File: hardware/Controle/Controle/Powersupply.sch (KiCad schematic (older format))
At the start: 14 parts, among them U401 AMS1117-3.3, U402 AMS1117-5, U403 K78L15-1000R3

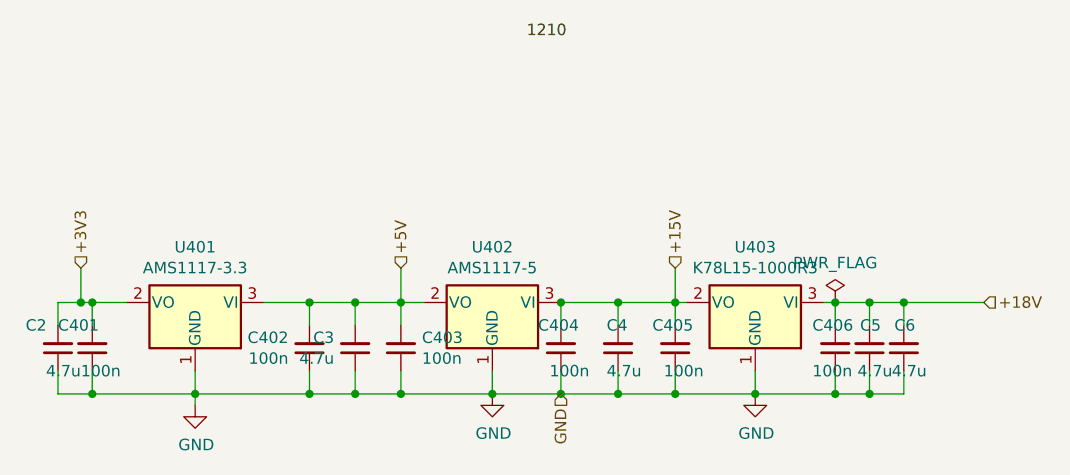
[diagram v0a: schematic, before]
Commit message: first version of layout
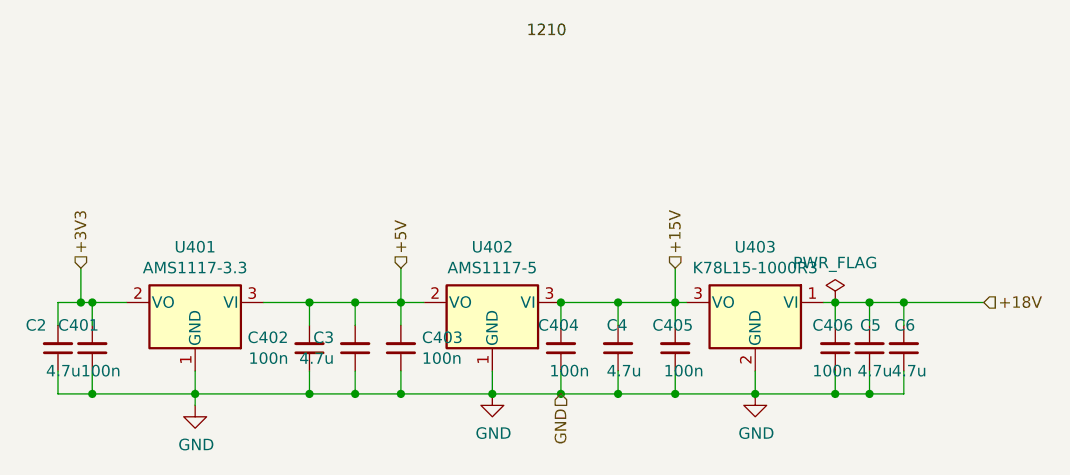
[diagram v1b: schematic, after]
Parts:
- removed U403: K78L15-1000R3, KicadZeniteSolarLibrary18:TO-220-3_Horizontal_TabDown_SMD, symbol Regulator_Linear:AP1117-15
- added U403: K78L15-1000R3, KicadZeniteSolarLibrary18:TO-220-3_Horizontal_Tabless_SMD, symbol Regulator_Linear:LM7805_TO220
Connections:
- net +15V: now also U403.3 (VO)
- net +18V: now also U403.1 (VI)
- net GND: now also U403.2 (GND)
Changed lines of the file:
@@
 GND
-$Comp
-L Regulator_Linear:AP1117-15 U403
-U 1 1 608AFF81
-P 7600 3700
-F 0 "U403" H 7600 3942 50  0000 C CNN
-F 1 "K78L15-1000R3" H 7600 3851 50  0000 C CNN
-F 2 "KicadZeniteSolarLibrary18:TO-220-3_Horizontal_TabDown_SMD" H 7600 3900 50  0001 C CNN
-F 3 "" H 7700 3450 50  0001 C CNN
-	1    7600 3700
-	-1   0    0    -1
-$EndComp
 $Comp
 L Device:C_Small C?
@@
 Text Label 6600 2550 0    50   ~ 0
 1210
+$Comp
+L Regulator_Linear:LM7805_TO220 U403
+U 1 1 609F70B2
+P 7600 3700
+F 0 "U403" H 7600 3942 50  0000 C CNN
+F 1 "K78L15-1000R3" H 7600 3851 50  0000 C CNN
+F 2 "KicadZeniteSolarLibrary18:TO-220-3_Horizontal_Tabless_SMD" H 7600 3925 50  0001 C CIN
+F 3 "https://www.onsemi.cn/PowerSolutions/document/MC7800-D.PDF" H 7600 3650 50  0001 C CNN
+	1    7600 3700
+	-1   0    0    -1
+$EndComp
 $EndSCHEMATC

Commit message: falta acabamento
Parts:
- C2, C3, C4, C5, C6: footprint Capacitor_SMD:C_1210_3225Metric_Pad1.33x2.70mm_HandSolder -> Capacitor_SMD:C_1206_3216Metric_Pad1.33x1.80mm_HandSolder
- U401: footprint Package_TO_SOT_SMD:SOT-223-3_TabPin2 -> Package_TO_SOT_SMD:SOT-89-3
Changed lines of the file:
@@
 F 0 "U401" H 5150 3942 50  0000 C CNN
 F 1 "AMS1117-3.3" H 5150 3851 50  0000 C CNN
-F 2 "Package_TO_SOT_SMD:SOT-223-3_TabPin2" H 5150 3900 50  0001 C CNN
+F 2 "Package_TO_SOT_SMD:SOT-89-3" H 5150 3900 50  0001 C CNN
 F 3 "" H 5250 3450 50  0001 C CNN
 	1    5150 3700
@@
 F 0 "C3" H 5758 3854 50  0000 R CNN
 F 1 "4.7u" H 5758 3945 50  0000 R CNN
-F 2 "Capacitor_SMD:C_1210_3225Metric_Pad1.33x2.70mm_HandSolder" H 5850 3900 50  0001 C CNN
+F 2 "Capacitor_SMD:C_1206_3216Metric_Pad1.33x1.80mm_HandSolder" H 5850 3900 50  0001 C CNN
 F 3 "~" H 5850 3900 50  0001 C CNN
 	1    5850 3900
@@
 F 0 "C2" H 4500 3800 50  0000 R CNN
 F 1 "4.7u" H 4650 4000 50  0000 R CNN
-F 2 "Capacitor_SMD:C_1210_3225Metric_Pad1.33x2.70mm_HandSolder" H 4550 3900 50  0001 C CNN
+F 2 "Capacitor_SMD:C_1206_3216Metric_Pad1.33x1.80mm_HandSolder" H 4550 3900 50  0001 C CNN
 F 3 "~" H 4550 3900 50  0001 C CNN
 	1    4550 3900
@@
 F 0 "C5" H 8150 3800 50  0000 R CNN
 F 1 "4.7u" H 8200 4000 50  0000 R CNN
-F 2 "Capacitor_SMD:C_1210_3225Metric_Pad1.33x2.70mm_HandSolder" H 8100 3900 50  0001 C CNN
+F 2 "Capacitor_SMD:C_1206_3216Metric_Pad1.33x1.80mm_HandSolder" H 8100 3900 50  0001 C CNN
 F 3 "~" H 8100 3900 50  0001 C CNN
 	1    8100 3900
@@
 F 0 "C4" H 7050 3800 50  0000 R CNN
 F 1 "4.7u" H 7050 4000 50  0000 R CNN
-F 2 "Capacitor_SMD:C_1210_3225Metric_Pad1.33x2.70mm_HandSolder" H 7000 3900 50  0001 C CNN
+F 2 "Capacitor_SMD:C_1206_3216Metric_Pad1.33x1.80mm_HandSolder" H 7000 3900 50  0001 C CNN
 F 3 "~" H 7000 3900 50  0001 C CNN
 	1    7000 3900
@@
 F 0 "C6" H 8300 3800 50  0000 R CNN
 F 1 "4.7u" H 8350 4000 50  0000 R CNN
-F 2 "Capacitor_SMD:C_1210_3225Metric_Pad1.33x2.70mm_HandSolder" H 8250 3900 50  0001 C CNN
+F 2 "Capacitor_SMD:C_1206_3216Metric_Pad1.33x1.80mm_HandSolder" H 8250 3900 50  0001 C CNN
 F 3 "~" H 8250 3900 50  0001 C CNN
 	1    8250 3900
